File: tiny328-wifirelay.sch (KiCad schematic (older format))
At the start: 8 parts, among them P1 RX868SH-DV, U1 TINY328, U2 ESP-01v090, U3 LD1117S33TR

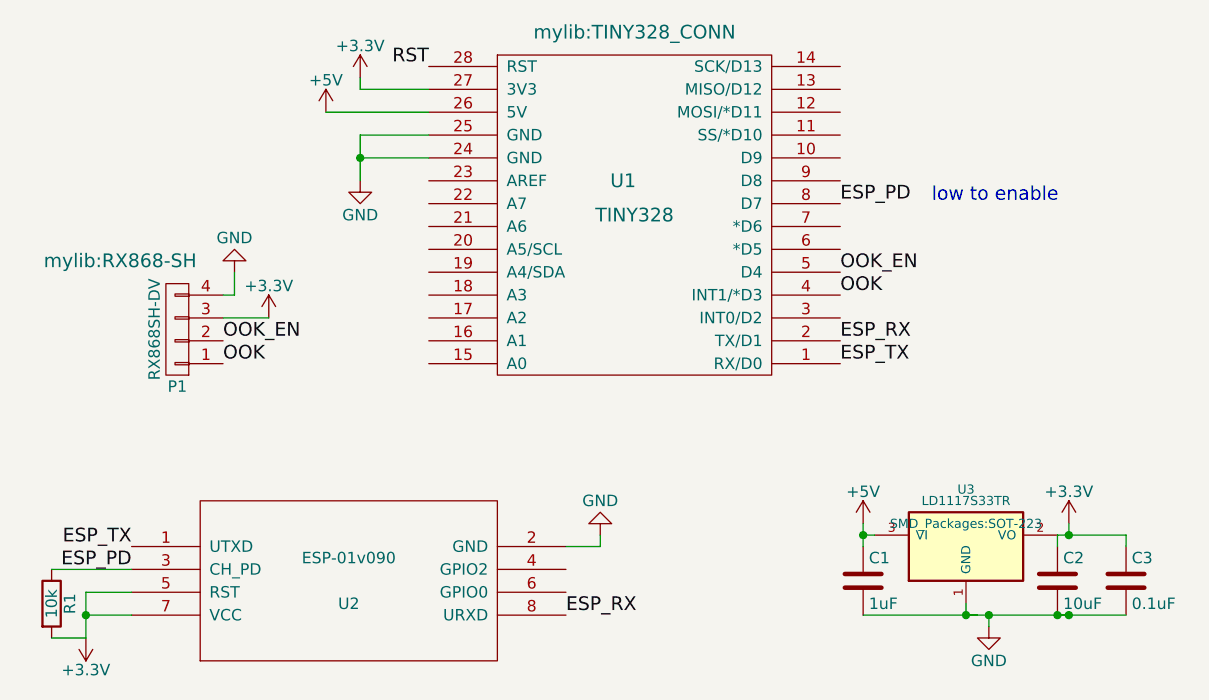
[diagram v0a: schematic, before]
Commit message: updated for PCB run #1
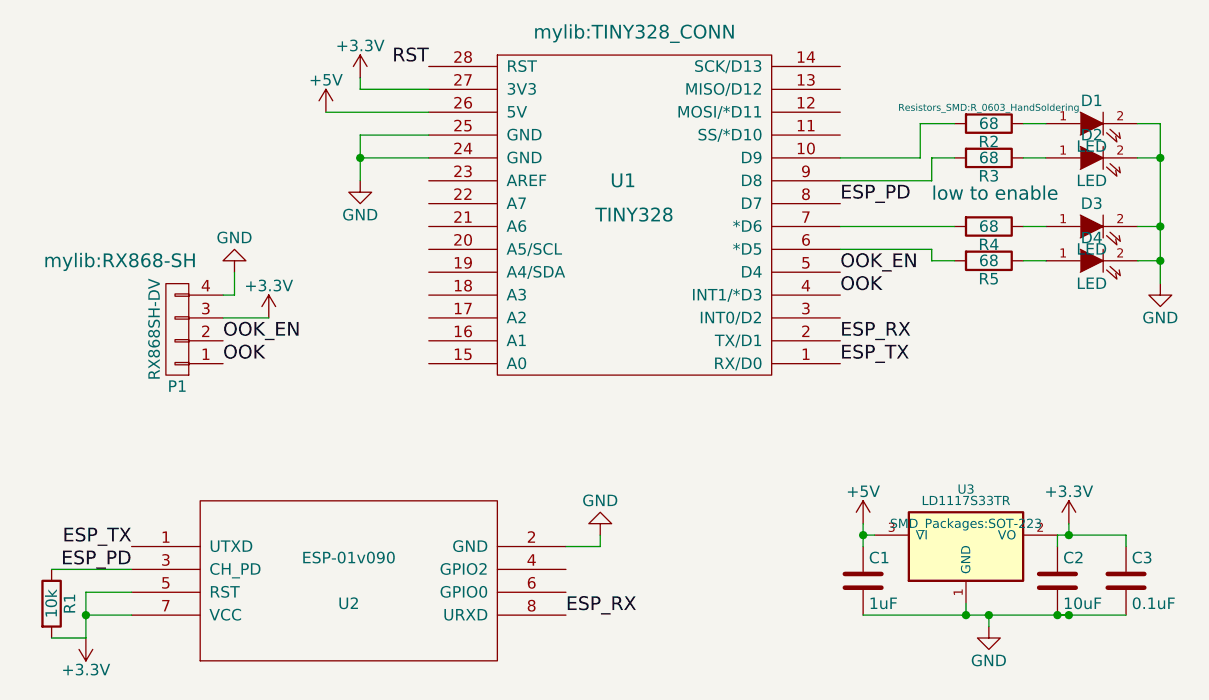
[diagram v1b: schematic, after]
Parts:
- added D1, D2, D3, D4: LED, LEDs:LED-0805, symbol LED
- added R2, R3, R4, R5: 68, Resistors_SMD:R_0603_HandSoldering, symbol R
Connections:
- wire segments 27 -> 45
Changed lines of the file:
@@
 Connection ~ 5450 3050
 Wire Wire Line
-	5700 3400 5000 3400
-Wire Wire Line
-	5050 3400 4550 3400
+	4550 3400 5700 3400
 Connection ~ 5000 3400
 Wire Wire Line
@@
 Connection ~ 5400 3400
 Connection ~ 5450 3400
+$Comp
+L R R5
+U 1 1 55E88AAB
+P 5100 1850
+F 0 "R5" V 5180 1850 50  0000 C CNN
+F 1 "68" V 5100 1850 50  0000 C CNN
+F 2 "Resistors_SMD:R_0603_HandSoldering" V 5030 1850 30  0001 C CNN
+F 3 "" H 5100 1850 30  0000 C CNN
+	1    5100 1850
+	0    1    1    0
+$EndComp
+$Comp
+L R R4
+U 1 1 55E88AED
+P 5100 1700
+F 0 "R4" V 5180 1700 50  0000 C CNN
+F 1 "68" V 5100 1700 50  0000 C CNN
+F 2 "Resistors_SMD:R_0603_HandSoldering" V 5030 1700 30  0001 C CNN
+F 3 "" H 5100 1700 30  0000 C CNN
+	1    5100 1700
+	0    1    1    0
+$EndComp
+$Comp
+L R R3
+U 1 1 55E88B16
+P 5100 1400
+F 0 "R3" V 5180 1400 50  0000 C CNN
+F 1 "68" V 5100 1400 50  0000 C CNN
+F 2 "Resistors_SMD:R_0603_HandSoldering" V 5030 1400 30  0001 C CNN
+F 3 "" H 5100 1400 30  0000 C CNN
+	1    5100 1400
+	0    1    1    0
+$EndComp
+$Comp
+L R R2
+U 1 1 55E88B3C
+P 5100 1250
+F 0 "R2" V 5180 1250 50  0000 C CNN
+F 1 "68" V 5100 1250 50  0000 C CNN
+F 2 "Resistors_SMD:R_0603_HandSoldering" V 5030 1250 30  0000 C CNN
+F 3 "" H 5100 1250 30  0000 C CNN
+	1    5100 1250
+	0    1    1    0
+$EndComp
+$Comp
+L LED D1
+U 1 1 55E88D78
+P 5550 1250
+F 0 "D1" H 5550 1350 50  0000 C CNN
+F 1 "LED" H 5550 1150 50  0000 C CNN
+F 2 "LEDs:LED-0805" H 5550 1250 60  0001 C CNN
+F 3 "" H 5550 1250 60  0000 C CNN
+	1    5550 1250
+	1    0    0    -1
+$EndComp
+$Comp
+L LED D2
+U 1 1 55E88DA6
+P 5550 1400
+F 0 "D2" H 5550 1500 50  0000 C CNN
+F 1 "LED" H 5550 1300 50  0000 C CNN
+F 2 "LEDs:LED-0805" H 5550 1400 60  0001 C CNN
+F 3 "" H 5550 1400 60  0000 C CNN
+	1    5550 1400
+	1    0    0    -1
+$EndComp
+$Comp
+L LED D3
+U 1 1 55E88DCB
+P 5550 1700
+F 0 "D3" H 5550 1800 50  0000 C CNN
+F 1 "LED" H 5550 1600 50  0000 C CNN
+F 2 "LEDs:LED-0805" H 5550 1700 60  0001 C CNN
+F 3 "" H 5550 1700 60  0000 C CNN
+	1    5550 1700
+	1    0    0    -1
+$EndComp
+$Comp
+L LED D4
+U 1 1 55E88DF3
+P 5550 1850
+F 0 "D4" H 5550 1950 50  0000 C CNN
+F 1 "LED" H 5550 1750 50  0000 C CNN
+F 2 "LEDs:LED-0805" H 5550 1850 60  0001 C CNN
+F 3 "" H 5550 1850 60  0000 C CNN
+	1    5550 1850
+	1    0    0    -1
+$EndComp
+Wire Wire Line
+	4450 1800 4850 1800
+Wire Wire Line
+	4850 1800 4850 1850
+Wire Wire Line
+	4850 1850 4950 1850
+Wire Wire Line
+	4950 1700 4450 1700
+Wire Wire Line
+	5250 1700 5350 1700
+Wire Wire Line
+	5250 1850 5350 1850
+Wire Wire Line
+	5250 1400 5350 1400
+Wire Wire Line
+	4450 1500 4850 1500
+Wire Wire Line
+	4850 1500 4850 1400
+Wire Wire Line
+	4850 1400 4950 1400
+Wire Wire Line
+	4950 1250 4800 1250
+Wire Wire Line
+	4800 1250 4800 1400
+Wire Wire Line
+	4800 1400 4450 1400
+Wire Wire Line
+	5250 1250 5350 1250
+$Comp
+L GND #PWR011
+U 1 1 55E891D2
+P 5850 1950
+F 0 "#PWR011" H 5850 1700 50  0001 C CNN
+F 1 "GND" H 5850 1800 50  0000 C CNN
+F 2 "" H 5850 1950 60  0000 C CNN
+F 3 "" H 5850 1950 60  0000 C CNN
+	1    5850 1950
+	1    0    0    -1
+$EndComp
+Wire Wire Line
+	5750 1850 5850 1850
+Wire Wire Line
+	5850 1250 5850 1950
+Wire Wire Line
+	5750 1700 5850 1700
+Connection ~ 5850 1850
+Wire Wire Line
+	5750 1400 5850 1400
+Connection ~ 5850 1700
+Wire Wire Line
+	5750 1250 5850 1250
+Connection ~ 5850 1400
 $EndSCHEMATC
